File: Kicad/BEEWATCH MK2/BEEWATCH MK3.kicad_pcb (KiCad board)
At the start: 2 copper layers, 40.3 x 39.7 mm, 115 parts, among them IC1 LTC3549EDCB#TRMPBF, J1 USB_C_Receptacle_USB2.0, J3 Conn_02x06_Odd_Even, Q1 DMG6968U, Q2 DMG6968U, Q3 DMP1045U-7, Q4 DMG6968U, Q5 BSS138, Q6 BSS138, Q7 BSS138, Q8 DMP1045U-7, Q9 DMG6968U, SW1 TK-074-4, SW2 TK-074-4, U1 ESP32-S3, U3 MPU-6050, U4 MCP73832-2-OT, U5 ME6217C33M5G, U7 RYS8830, U8 S-1206B18-M3T1G, Y1 40MHz, Y2 32.768KHz

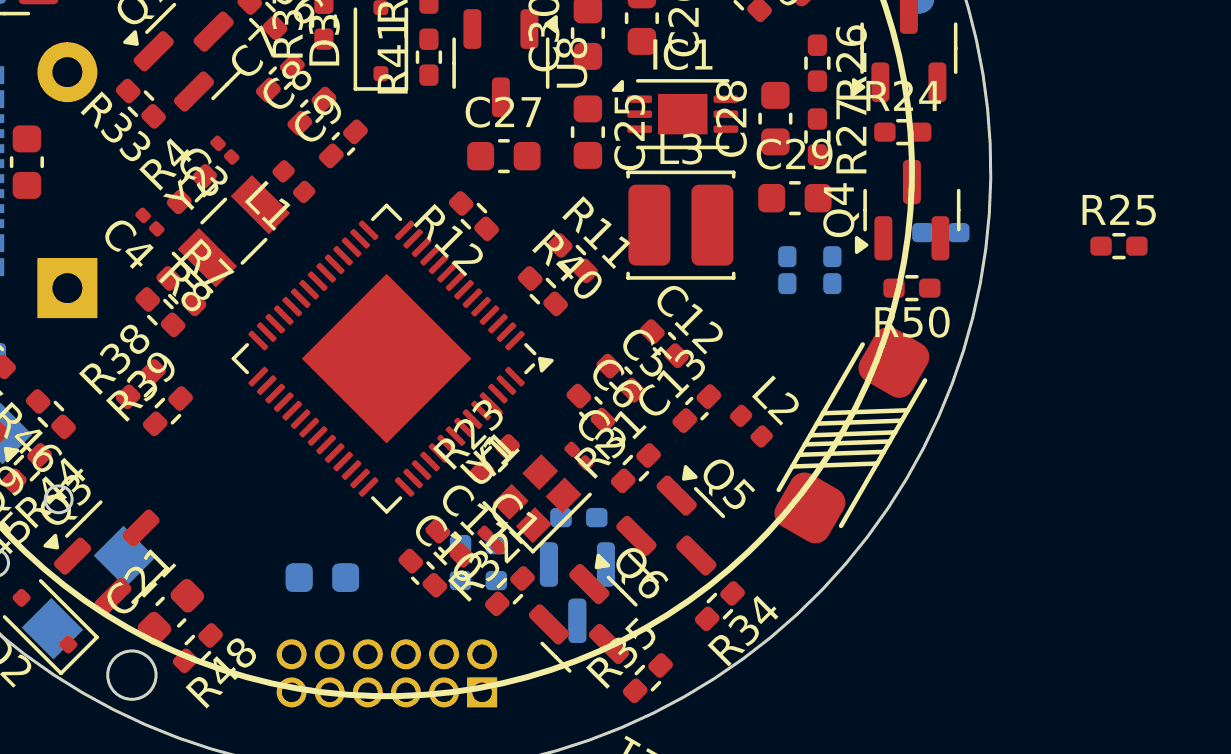
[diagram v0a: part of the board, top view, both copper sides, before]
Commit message: minor change in ESP32
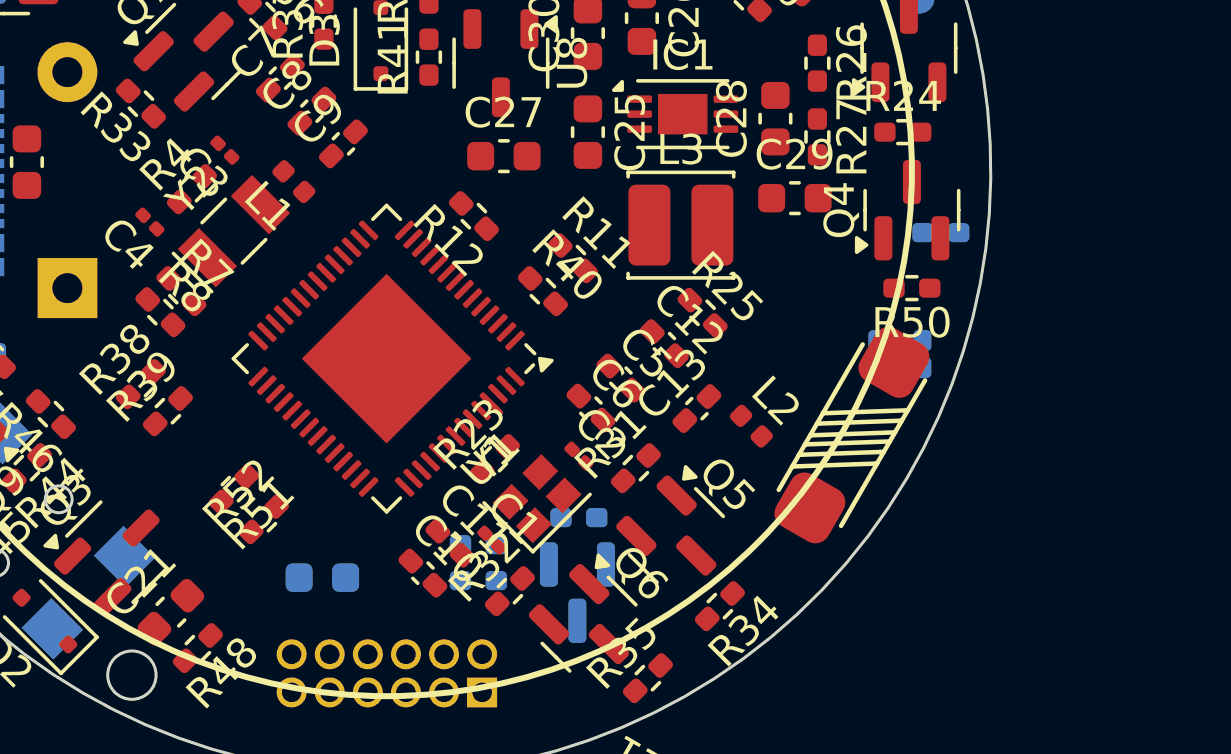
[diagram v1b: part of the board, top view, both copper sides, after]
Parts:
- added R51: 0, Resistor_SMD:R_0402_1005Metric_Pad0.72x0.64mm_HandSolder, F.Cu at (144.9, 115.6)
- added R52: 0, Resistor_SMD:R_0402_1005Metric_Pad0.72x0.64mm_HandSolder, F.Cu at (145.9, 116.6)
- U1: value ESP32-S3 -> ESP32-S3FH4R2
- moved R25 14.1 mm to (160.5, 109.7), turned to -45 degrees
- moved D1 4.10 mm to (167.1, 111.1)
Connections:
- U1 pad 51: unconnected-(U1-GPIO45-Pad51) -> Net-(U1-GPIO45)
- U1 pad 52: unconnected-(U1-GPIO46-Pad52) -> Net-(U1-GPIO46)
